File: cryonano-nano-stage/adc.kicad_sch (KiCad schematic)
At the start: 19 parts, among them U1 AD7124-8BCPZ-RL7, U6 LP5907MFX-3.3_NOPB

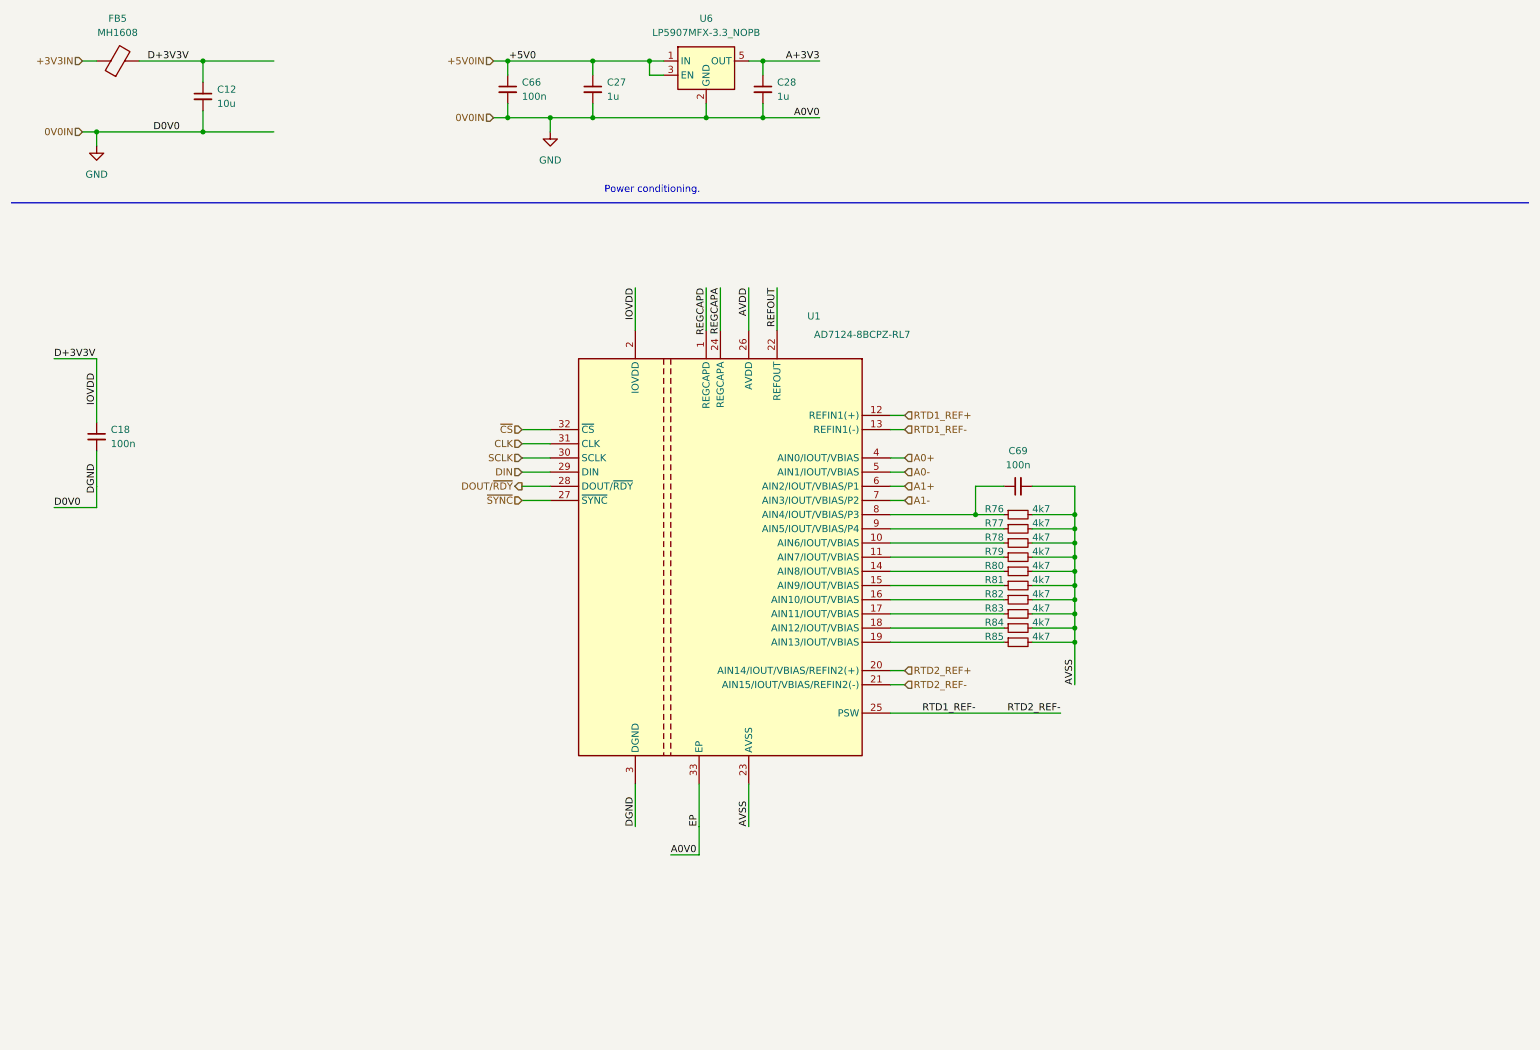
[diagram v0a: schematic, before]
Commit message: sch improved
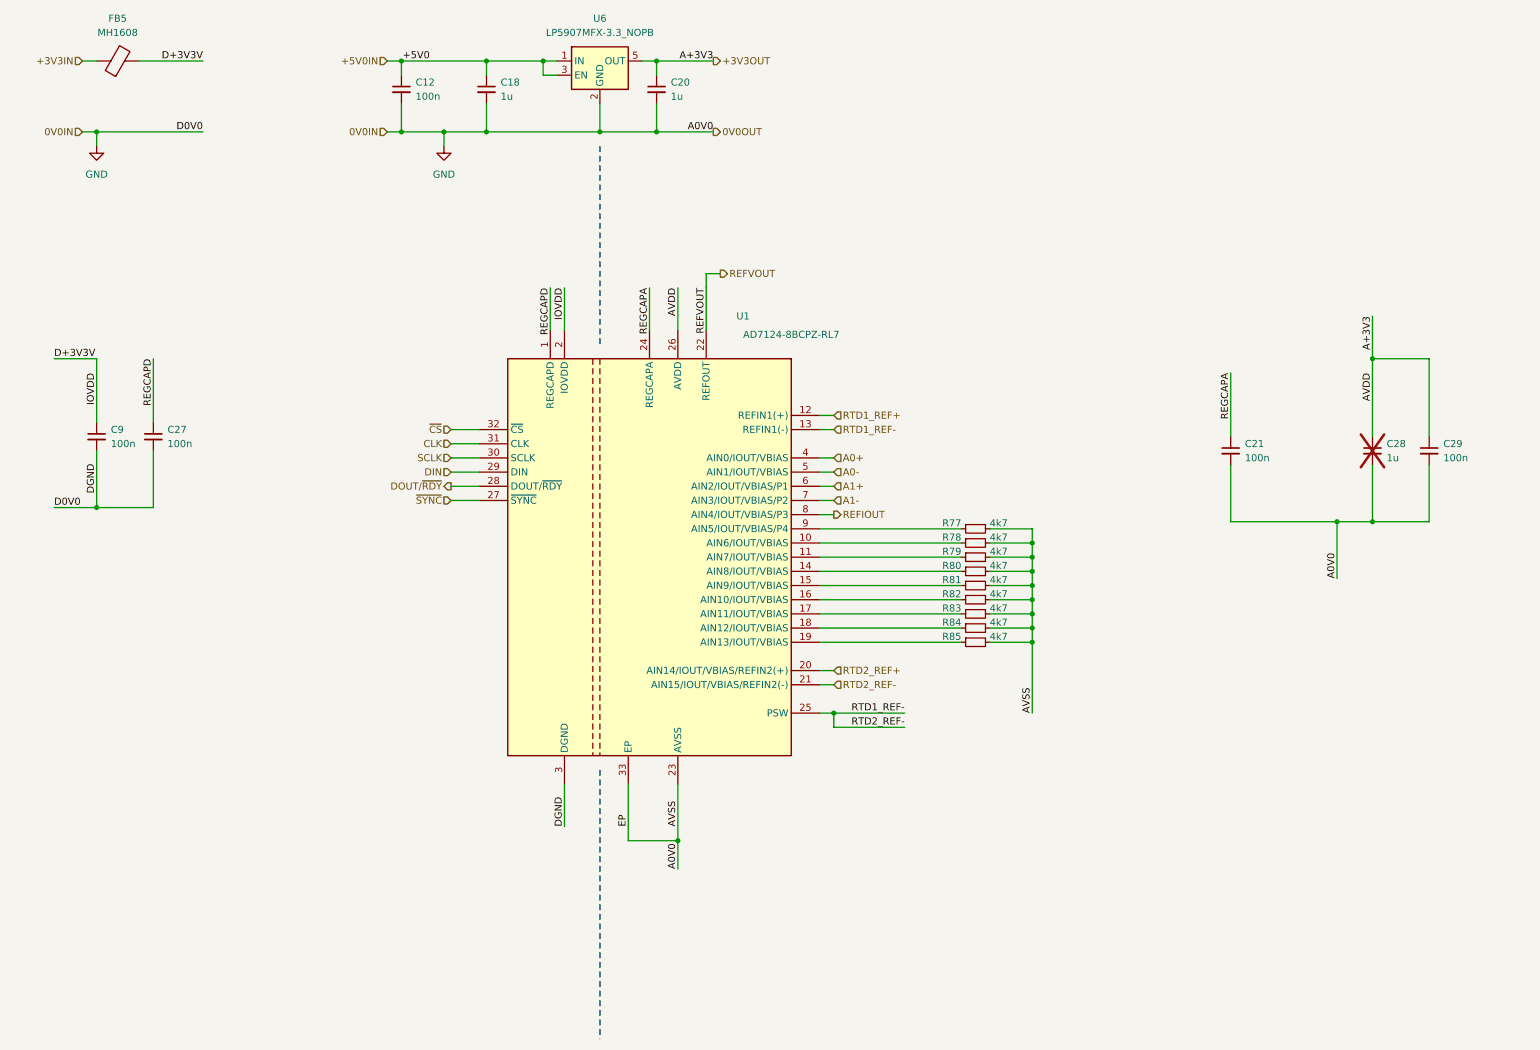
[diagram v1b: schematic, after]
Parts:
- removed C12: 10u, Capacitor_SMD:C_0805_2012Metric, symbol Device:C_Small
- removed C69: 100n, Capacitor_SMD:C_0603_1608Metric, symbol Device:C_Small
- removed R76: 4k7, Resistor_SMD:R_0603_1608Metric, symbol Device:R_Small
- added C21, C27, C29: 100n, Capacitor_SMD:C_0603_1608Metric, symbol Device:C_Small
- added C28: 1u, Capacitor_SMD:C_0603_1608Metric, symbol Device:C_Small
- renumbered C66 to C12, C27 to C18, C28 to C20, C18 to C9
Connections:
- net AVDD is gone; now on net +3V3OUT: U1.26 (AVDD)
- net AVSS is gone; now on net GND: R77.2, R78.2, R79.2, R80.2, R81.2, R82.2, R83.2, R84.2, R85.2, U1.23 (AVSS)
- net GND: now also C21.2, C27.2, C28.2, C29.2
- net REGCAPA: now also C21.1
- net REGCAPD: now also C27.1
- net REFIOUT: now reaches U1.8 (AIN4/IOUT/VBIAS/P3)
- net A+3V3 renamed +3V3OUT
- net +3V3OUT: now also C28.1, C29.1
- net REFOUT renamed REFVOUT
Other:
- note removed: "Power conditioning."
- moved on the sheet: C12, C18, C20, R77, R78, R79, R80, R81, R82, R83, R84, R85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
